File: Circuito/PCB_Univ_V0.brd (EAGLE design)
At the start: 97 x 54.9 mm, 21 parts

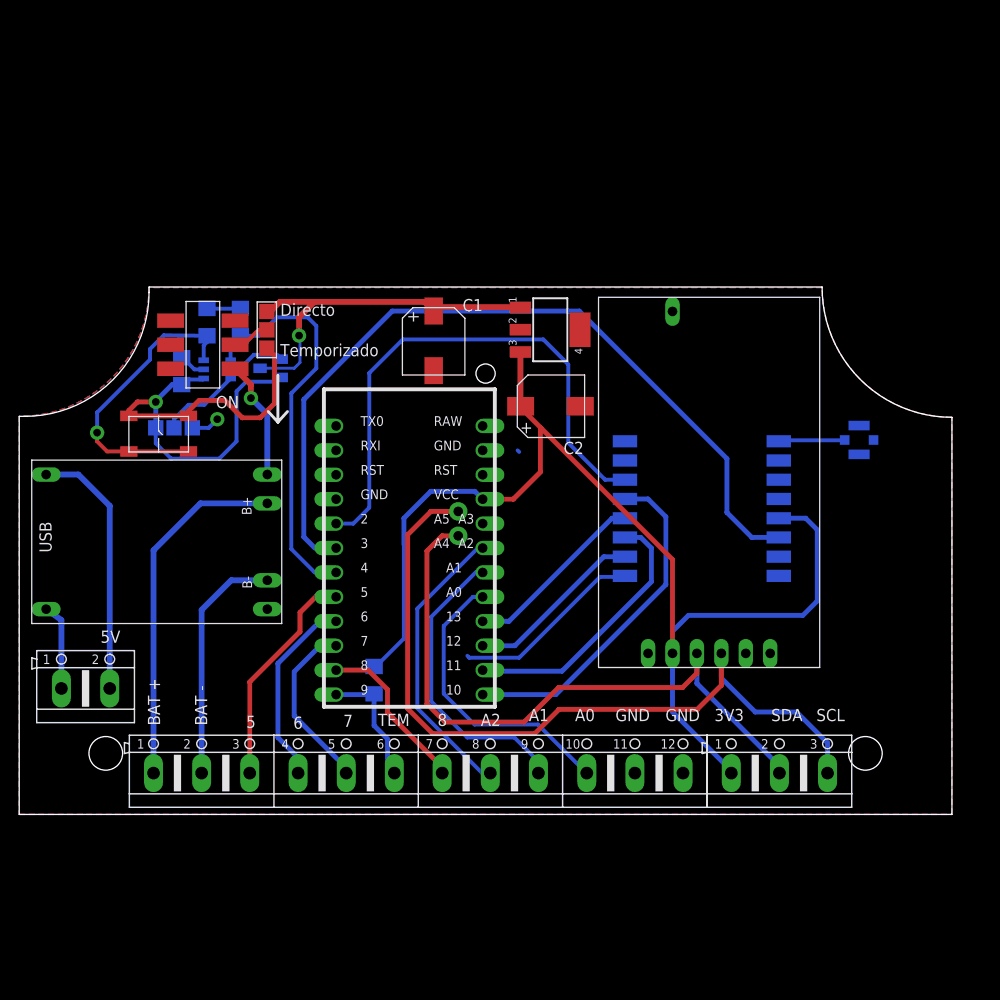
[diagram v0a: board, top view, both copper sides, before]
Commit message: Circuito V0
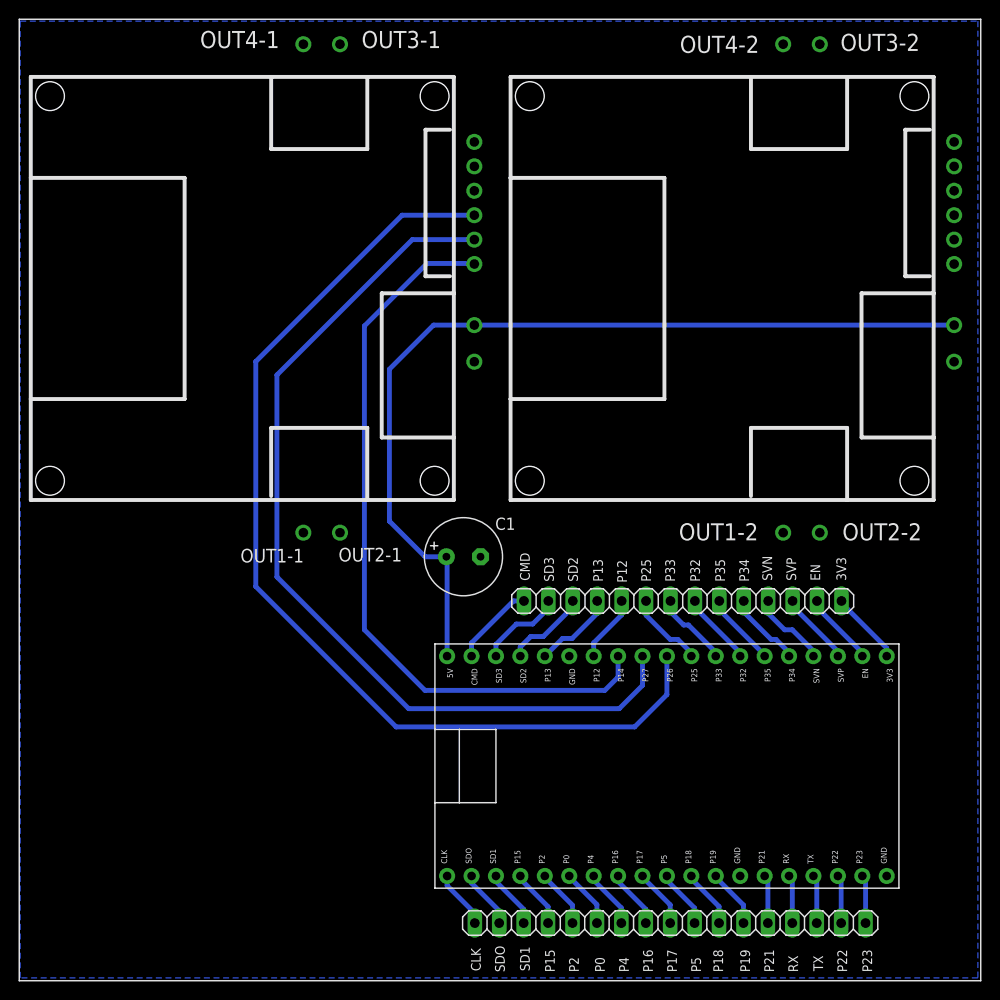
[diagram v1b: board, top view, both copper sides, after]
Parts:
- removed C2: 100uF, DAIMOB:CAP_SMD_100U
- removed C3: 100nF, rcl2:C1206
- removed R1: 4.7k, rcl:R1206
- removed R2: (no value), rcl:R1206
- removed R3: 10k, rcl:R1206
- removed U$10: SW_SMD, DAIMOB:SW_SMD
- removed U$11, U$12: JP_SMD, DAIMOB:JP_SMD
- removed U$3: RFM95W, DAIMOB:RFM95W
- removed U$4: MCP1826S-3302E/DB, DAIMOB:SOT223
- removed U$5: PMV250EPA, DAIMOB:SOT23-3
- removed U$6: SWITCH_SMD, DAIMOB:SWITCH_SMD
- removed U$7: ANTENA_IPX, DAIMOB:ANTENA_IPX
- removed U$8: CHARGER, DAIMOB:CHARGER
- removed U$9: RTC_DS3231, DAIMOB:RTC_DS2331
- removed X1: (no value), con-ptr500:AK500/2
- removed X2: (no value), con-ptr500:AK500/12
- removed X4: (no value), con-ptr500:AK500/3
- added ESP1: ESP12_MOD, DAIMOB:ESP32_MOD
- added JP1: (no value), pinhead:1X17
- added JP2: (no value), pinhead:1X14
- C1: value 100uF -> (none); device DAIMOB:CAP_SMD_100U -> rcl2:E3,5-8
- U$1: value PRO_MINI -> DRIVER_MOTOR; device DAIMOB:PRO_MINI -> DAIMOB:DRIVER_MOTOR
- U$2: value TPL5110 -> DRIVER_MOTOR; device DAIMOB:SOT23-6 -> DAIMOB:DRIVER_MOTOR
- moved U$2 53.3 mm to (73.1, 72.0), flipped to the top
- moved C1 18.9 mm to (46.2, 44.1), turned to 0 degrees
- moved U$1 17.3 mm to (23.2, 72.0), turned to 90 degrees
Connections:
- removed net 0V: U$8.IN-, X1.1
- removed net 5V: U$8.IN+, X1.2
- removed net A0: U$1.17, X2.10
- removed net A1: U$1.18, X2.9
- removed net A2: U$1.19, X2.8
- removed net ANT: U$3.1, U$7.1
- removed net BAT+: U$8.B+, X2.1
- removed net BAT-: U$8.B-, X2.2
- removed net DELAY: R2.2, U$10.3, U$10.4, U$2.P$3
- removed net DONE: R3.2, U$1.7, U$2.P$4
- removed net DRV: U$2.P$5, U$5.1
- removed net EN: U$12.P$2, U$2.P$6
- removed net GPIO0: U$1.6, U$3.6
- removed net IO5: U$1.8, X2.3
- removed net IO6: U$1.9, X2.4
- removed net IO7: U$1.10, X2.5
- removed net IO8: U$1.11, X2.7
- removed net MISO: U$1.15, U$3.10
- removed net MOSI: U$1.14, U$3.11
- removed net NSS: U$1.13, U$3.13
- removed net OUT+: U$6.P$1, U$8.OUT+
- removed net OUT+1: U$11.P$2, U$6.P$2
- removed net RST: U$1.5, U$3.14
- removed net SCK: U$1.16, U$3.12
- removed net SCL: U$1.22, U$9.SCL, X4.3
- removed net SDA: U$1.20, U$9.SDA, X4.2
- removed net TEMP: R1.1, U$1.12, X2.6
- removed net VDD: C3.1, U$10.1, U$10.2, U$11.P$3, U$12.P$3, U$2.P$1, U$5.2
- removed net VIN: C1.2+, U$11.P$1, U$4.1, U$5.3
- new net N$1: ESP1.P$30, U$1.N1
- new net N$10: ESP1.P$27, JP2.7
- new net N$11: ESP1.P$26, JP2.8
- new net N$12: ESP1.P$25, JP2.9
- new net N$13: ESP1.P$24, JP2.10
- new net N$14: ESP1.P$23, JP2.11
- new net N$15: ESP1.P$22, JP2.12
- new net N$16: ESP1.P$21, JP2.13
- new net N$17: ESP1.P$20, JP2.14
- new net N$18: ESP1.P$18, JP1.1
- new net N$19: ESP1.P$17, JP1.2
- new net N$2: ESP1.P$29, U$1.N2
- new net N$20: ESP1.P$16, JP1.3
- new net N$21: ESP1.P$15, JP1.4
- new net N$22: ESP1.P$14, JP1.5
- new net N$23: ESP1.P$12, JP1.6
- new net N$24: ESP1.P$11, JP1.7
- new net N$25: ESP1.P$10, JP1.8
- new net N$26: ESP1.P$9, JP1.9
- new net N$27: ESP1.P$8, JP1.10
- new net N$28: ESP1.P$7, JP1.11
- new net N$29: ESP1.P$6, JP1.12
- new net N$3: ESP1.P$31, U$1.ENA
- new net N$30: ESP1.P$5, JP1.13
- new net N$31: ESP1.P$4, JP1.14
- new net N$32: ESP1.P$3, JP1.15
- new net N$33: ESP1.P$2, JP1.16
- new net N$34: ESP1.P$1, JP1.17
- new net N$4: ESP1.P$37, JP2.1
- new net N$5: ESP1.P$36, JP2.2
- new net N$6: ESP1.P$35, JP2.3
- new net N$7: ESP1.P$34, JP2.4
- new net N$8: ESP1.P$32, JP2.5
- new net N$9: ESP1.P$28, JP2.6
- net GND: now also C1.-, ESP1.P$13, ESP1.P$19, ESP1.P$33, U$1.GND, U$2.GND; no longer C1.1-, C2.1-, C3.2, R2.1, R3.1, U$1.25, U$1.4, U$12.P$1, U$2.P$2, U$3.16, U$3.2, U$3.9, U$4.2, U$4.4, U$7.2, U$7.3, U$7.4, U$8.OUT-, U$9.GND, U$9.GND@1, X2.11, X2.12
- net VCC: now also C1.+, ESP1.P$38, U$1.5V, U$2.5V; no longer C2.2+, R1.2, U$1.23, U$3.5, U$4.3, U$9.VCC, X4.1
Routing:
- net N$2: track 0.00 -> 106.6 mm
- net N$1: track 0.00 -> 95.1 mm
- net GPIO0: track 84.4 -> 0.00 mm
- net SCL: track 83.0 -> 0.00 mm
- net N$3: track 0.00 -> 77.5 mm
- net SDA: track 68.9 -> 0.00 mm
- net VDD: track 57.9 -> 0.00 mm, vias 1 -> 0
- net RST: track 57.0 -> 0.00 mm
- net DONE: track 42.0 -> 0.00 mm
- net VIN: track 38.8 -> 0.00 mm, vias 1 -> 0
- net BAT+: track 37.0 -> 0.00 mm
- net NSS: track 35.9 -> 0.00 mm
- net DELAY: track 31.0 -> 0.00 mm, vias 1 -> 0
- net A1: track 31.0 -> 0.00 mm
- net A0: track 30.6 -> 0.00 mm
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- removed copper zone on layer 1, net GND
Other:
- board size 97 x 54.9 mm -> 100 x 100 mm
- board text added: "CLK"
- board text added: "CMD"
- board text added: "EN"
- board text added: "OUT1-1"
- board text added: "OUT1-2"
- board text added: "OUT2-1"
- board text added: "OUT2-2"
- board text added: "OUT3-1"
- board text added: "OUT3-2"
- board text added: "OUT4-1"
- board text added: "OUT4-2"
- board text added: "P0"
- board text added: "P12"
- board text added: "P13"
- board text added: "P15"
- board text added: "P16"
- board text added: "P17"
- board text added: "P18"
- board text added: "P19"
- board text added: "P2"
- board text added: "P21"
- board text added: "P22"
- board text added: "P23"
- board text added: "P25"
- board text added: "P32"
- board text added: "P33"
- board text added: "P34"
- board text added: "P35"
- board text added: "P4"
- board text added: "P5"
- board text added: "RX"
- board text added: "SD1"
- board text added: "SD2"
- board text added: "SD3"
- board text added: "SDO"
- board text added: "SVN"
- board text added: "SVP"
- board text added: "TX"
- board text removed: "5"
- board text removed: "5V"
- board text removed: "6"
- board text removed: "7"
- board text removed: "8"
- board text removed: "A0"
- board text removed: "A1"
- board text removed: "A2"
- board text removed: "BAT +"
- board text removed: "BAT -"
- board text removed: "Directo"
- board text removed: "GND"
- board text removed: "ON"
- board text removed: "SCL"
- board text removed: "SDA"
- board text removed: "TEM"
- board text removed: "Temporizado"
